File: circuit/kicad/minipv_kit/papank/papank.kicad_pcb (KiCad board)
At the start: 2 copper layers, 58.3 x 31.7 mm, 18 parts, among them SW1 SW_DIP_x04

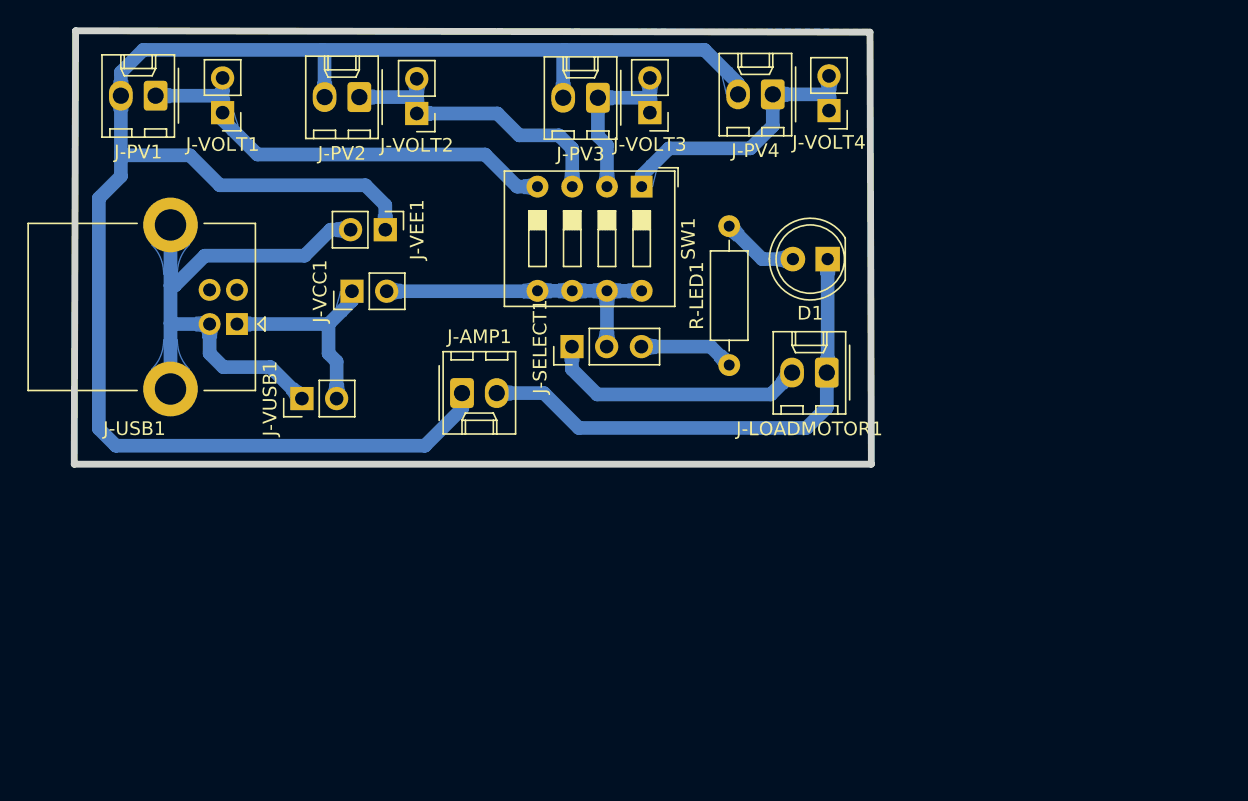
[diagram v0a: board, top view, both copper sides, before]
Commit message: PCB Mini PV
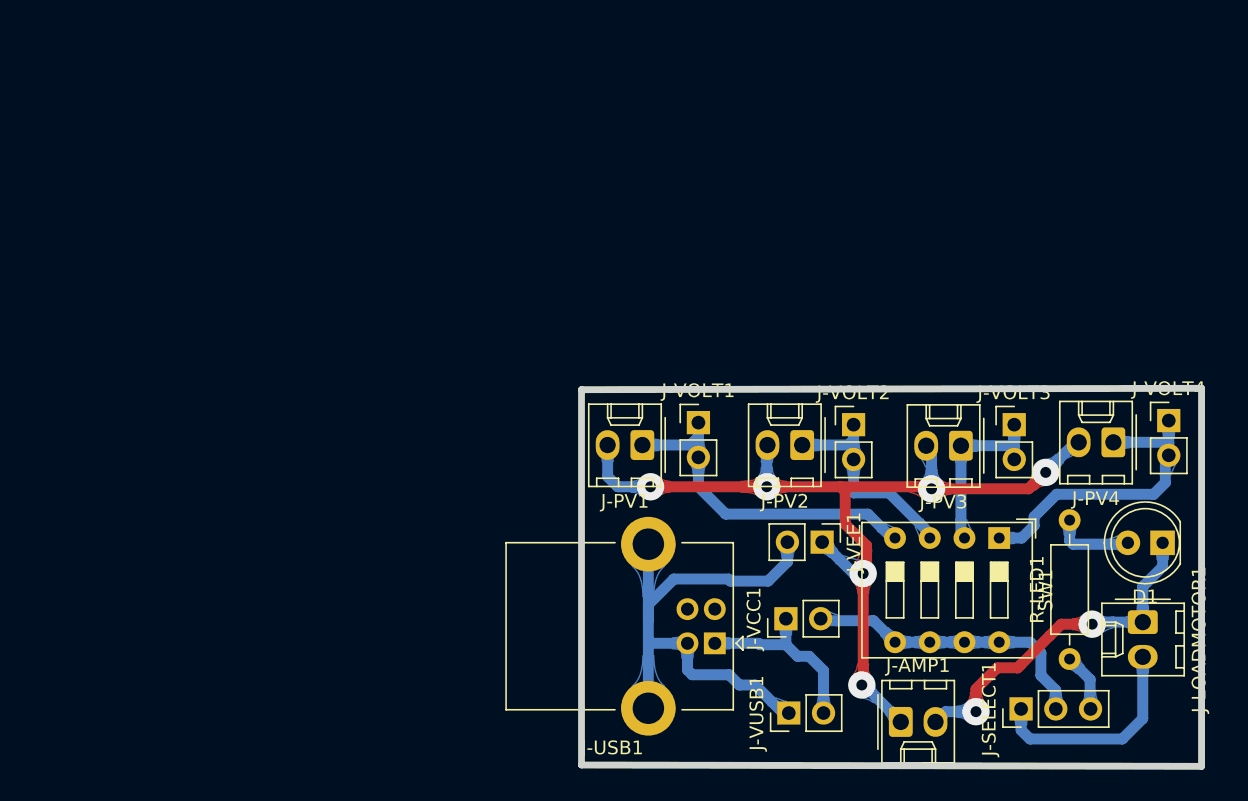
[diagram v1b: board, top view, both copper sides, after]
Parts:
- moved J-PV1 43.8 mm to (111.5, 72.4)
- moved J-VUSB1 42.4 mm to (122.3, 92.0)
- moved J-SELECT1 42.2 mm to (139.2, 91.7)
- moved J-USB1 42.0 mm to (116.8, 86.9)
- moved J-VOLT1 41.5 mm to (115.7, 70.8), turned to 0 degrees
- moved J-PV2 41.2 mm to (123.2, 72.4)
- moved J-AMP1 40.1 mm to (130.4, 92.7)
- moved J-VCC1 39.8 mm to (122.0, 85.1)
- moved J-VEE1 39.3 mm to (124.7, 79.5)
- moved J-VOLT2 39.2 mm to (127.0, 70.9), turned to 0 degrees
- moved J-PV3 36.8 mm to (134.8, 72.5)
- moved SW1 36.7 mm to (137.7, 79.2)
- moved J-PV4 35.6 mm to (146.0, 72.2)
- moved J-VOLT3 35.1 mm to (138.8, 70.9), turned to 0 degrees
- moved J-VOLT4 33.6 mm to (150.1, 70.6), turned to 0 degrees
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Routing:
- net GND: track 133.4 -> 68.3 mm, vias 0 -> 6
- net /LOAD_GND: track 36.7 -> 25.6 mm, vias 0 -> 2
- net /PV1: track 33.2 -> 25.0 mm
- net /PV2: track 22.0 -> 16.0 mm
- net /LOAD_LED: track 6.98 -> 4.28 mm
- net /LOAD_MOTOR: track 19.2 -> 16.6 mm
- net /PV4: track 20.9 -> 22.9 mm
- net VCC: track 15.5 -> 13.8 mm
- net /LOAD_VCC: track 22.8 -> 21.7 mm
- added copper zone on F.Cu, net (none)
- added copper zone on B.Cu, net GND
- removed copper zone on B.Cu, net (none)
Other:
- board size 58.3 x 31.7 mm -> 45.3 x 27.7 mm
